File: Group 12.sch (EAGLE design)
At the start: 13 parts

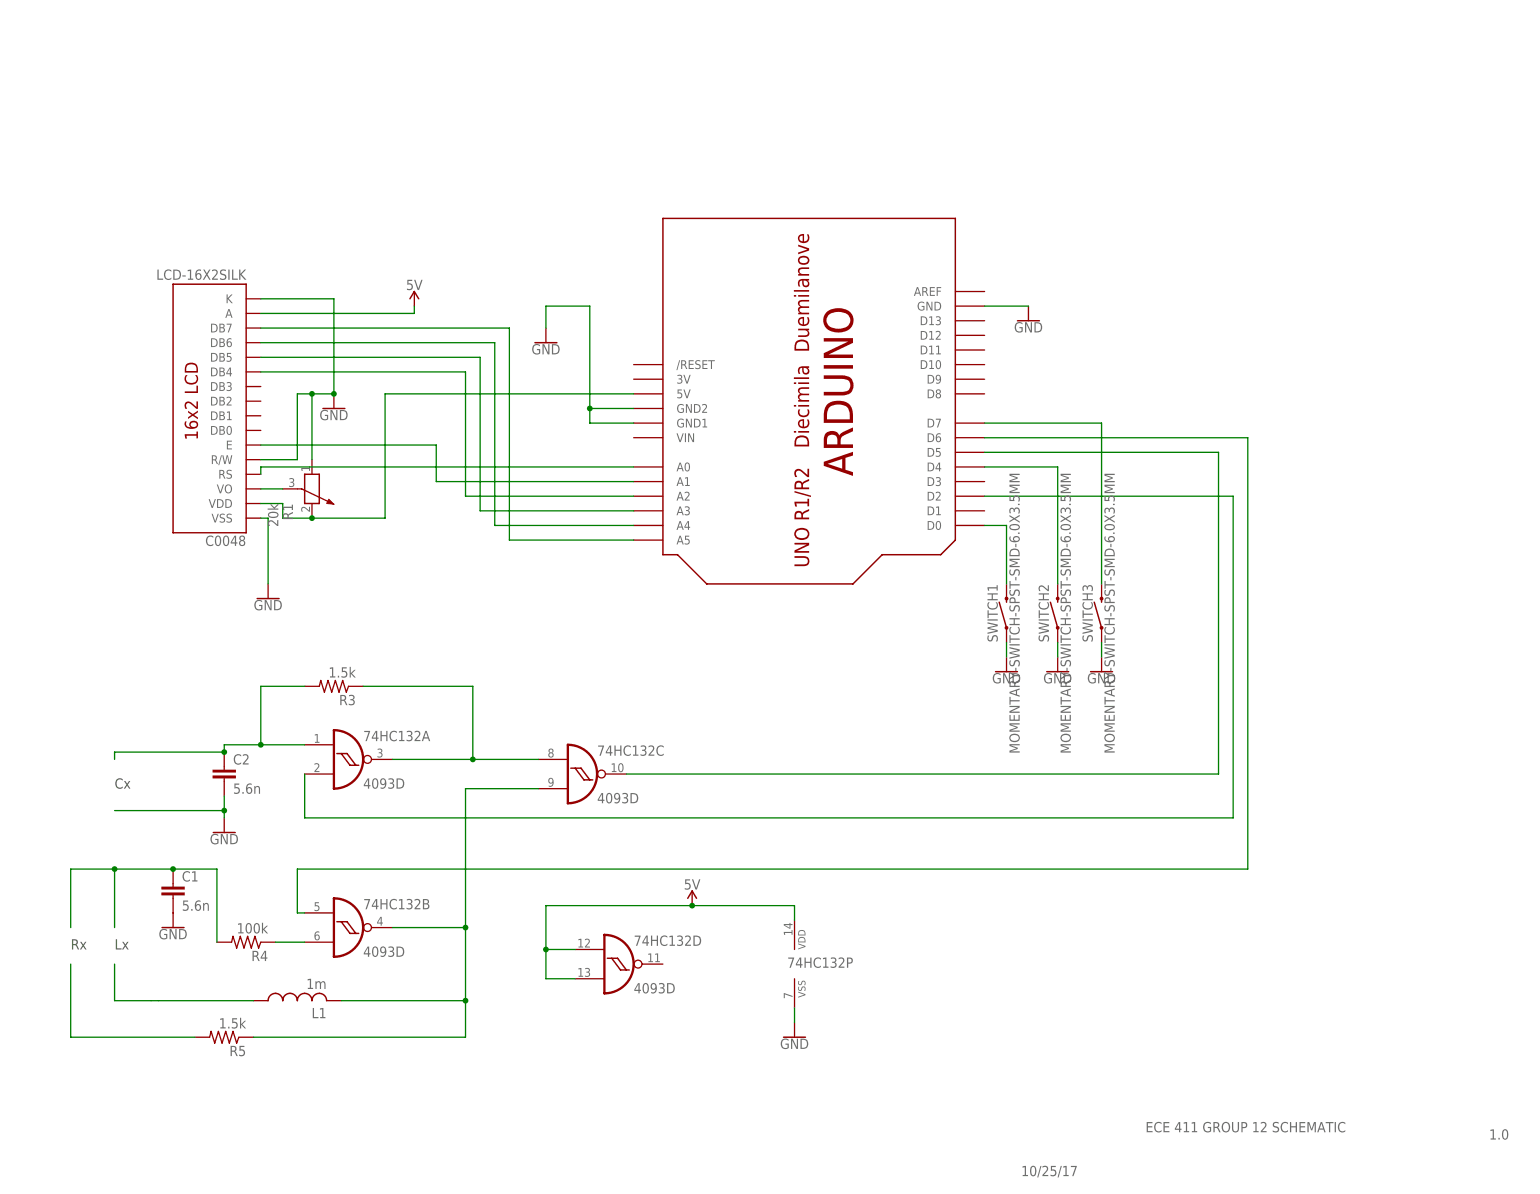
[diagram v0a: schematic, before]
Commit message: Schm and Proj Sch
Schematic and Project Schedule
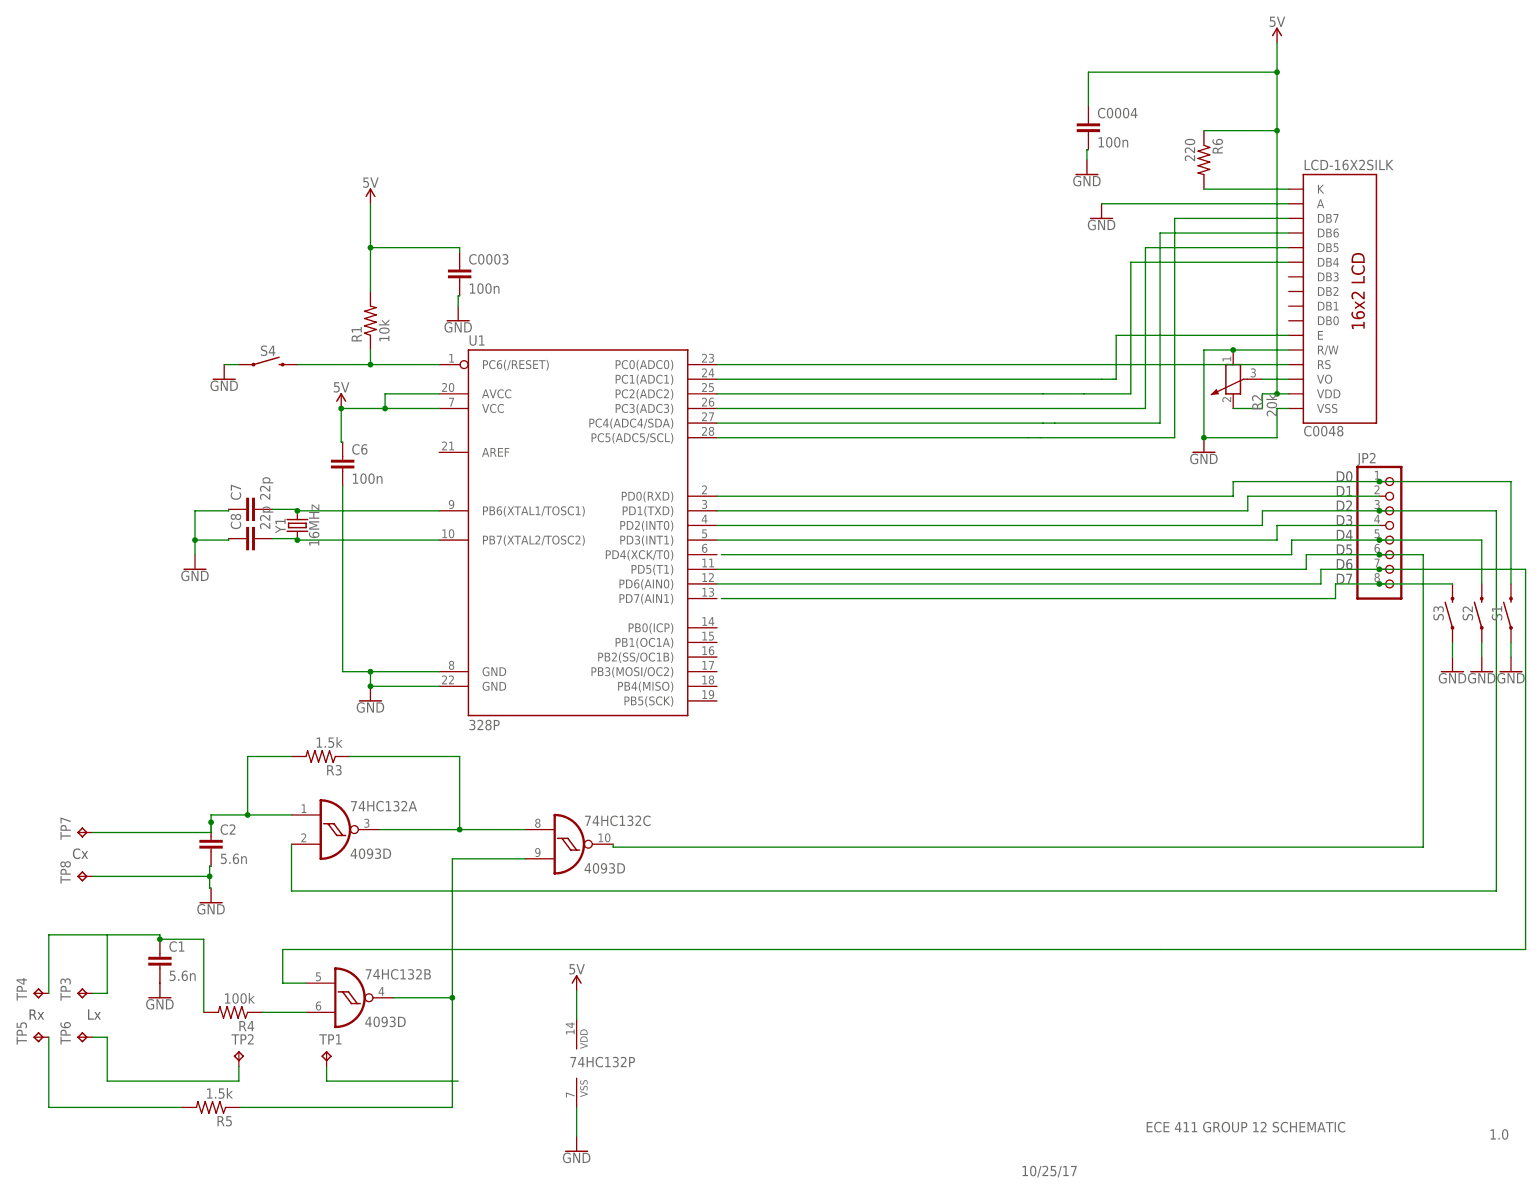
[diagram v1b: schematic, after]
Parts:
- removed L1: 1m, rcl:L-USL1812
- removed SWITCH1, SWITCH2, SWITCH3: MOMENTARY-SWITCH-SPST-SMD-6.0X3.5MM, SparkFun-Switches:MOMENTARY-SWITCH-SPST-SMD-6.0X3.5MM
- removed U$1: ARDUINOUNO, adafruit:ARDUINOUNO
- added C0003, C0004, C6: 100n, rcl:C-EUC0805K
- added C7, C8: 22p, rcl:C-EUC0805K
- added JP2: (no value), pinhead:PINHD-1X8
- added R2: 20k, rcl:POTENTIOMETER_PT-10
- added R6: 220, rcl:R-US_R0805
- added S1, S2, S3, S4: MOMENTARY-SWITCH-SPST-SMD-6.0X3.5MM, SparkFun-Switches:MOMENTARY-SWITCH-SPST-SMD-6.0X3.5MM
- added TP1, TP2, TP3, TP4, TP5, TP6, TP7, TP8: TPPAD1-13, testpad:TPPAD1-13
- added U1: 328P, SparkFun-IC-Microcontroller:ATMEGA328P_PDIP
- added Y1: 16MHz, SparkFun-Clocks:CRYSTAL-16MHZSMD-5X3.2
- R1: value 20k -> 10k; device rcl:POTENTIOMETER_PT_SPIN -> rcl:R-US_R0805
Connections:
- removed net N$19: SWITCH3.2, U$1.D7
- new net N$22: C0048.K, R6.2
- new net N$24: C7.2, U1.PB6(XTAL1/TOSC1), Y1.2
- new net N$25: C8.2, U1.PB7(XTAL2/TOSC2), Y1.1
- new net N$35: 74HC132C.O, JP2.6, U1.PD5(T1)
- new net N$36: JP2.4, U1.PD3(INT1)
- new net N$37: JP2.5, S2.2
- new net N$39: JP2.2, U1.PD1(TXD)
- new net N$40: JP2.1, S1.2, U1.PD0(RXD)
- net 5V: now also C0003.1, C0004.1, C0048.VDD, C6.1, R1.2, R2.2, R6.1, U1.AVCC, U1.VCC; no longer 74HC132D.I0, 74HC132D.I1, C0048.A
- net GND: now also C0003.2, C0004.2, C0048.A, C6.2, C7.1, C8.1, R2.1, S1.1, S2.1, S3.1, S4.1, TP8.TP, U1.GND@1, U1.GND@2; no longer C0048.K, R1.1, SWITCH1.1, SWITCH2.1, SWITCH3.1, U$1.GND, U$1.GND1, U$1.GND2
- net N$1: now also JP2.8, S3.2; no longer SWITCH1.2, U$1.D0
- net N$10: no longer L1.2
- net N$12: now also TP4.TP
- net N$13: now also TP1.TP; no longer 74HC132C.O, U$1.D5
- net N$14: now also TP2.TP, TP6.TP; no longer 74HC132B.I0, U$1.D6
- net N$15: now also R1.1, S4.2, U1.PC6(/RESET); no longer 74HC132A.I1, U$1.D2
- net N$16: now also TP3.TP; no longer L1.1
- net N$17: now also TP5.TP
- net N$18: now also 74HC132B.I0, JP2.7, U1.PD6(AIN0); no longer SWITCH2.2, U$1.D4
- net N$2: now also TP7.TP
- net N$20: now also R2.3; no longer R1.3
- net N$21: now also U1.PC0(ADC0); no longer U$1.A0
- net N$3: now also 74HC132A.I1, JP2.3, U1.PD2(INT0); no longer C0048.VDD, R1.2, U$1.5V
- net N$4: now also U1.PC1(ADC1); no longer U$1.A1
- net N$5: now also U1.PC2(ADC2); no longer U$1.A2
- net N$6: now also U1.PC3(ADC3); no longer U$1.A3
- net N$7: now also U1.PC4(ADC4/SDA); no longer U$1.A4
- net N$8: now also U1.PC5(ADC5/SCL); no longer U$1.A5
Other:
- note added: "D0"
- note added: "D1"
- note added: "D2"
- note added: "D3"
- note added: "D4"
- note added: "D5"
- note added: "D6"
- note added: "D7"
- moved on the sheet: 74HC132A, 74HC132B, 74HC132C, 74HC132P, C0048, C1, C2, R3, R4, R5
